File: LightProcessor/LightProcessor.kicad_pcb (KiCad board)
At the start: 2 copper layers, 78.5 x 80.8 mm, 30 parts, among them IC1 STM32G474RET6, J1 USB_C_Receptacle_USB2.0_16P, SW10 Tactile_6mm, U1 STLINK-V3MODS, U3 AP2112K-3.3, Y1 16MHz

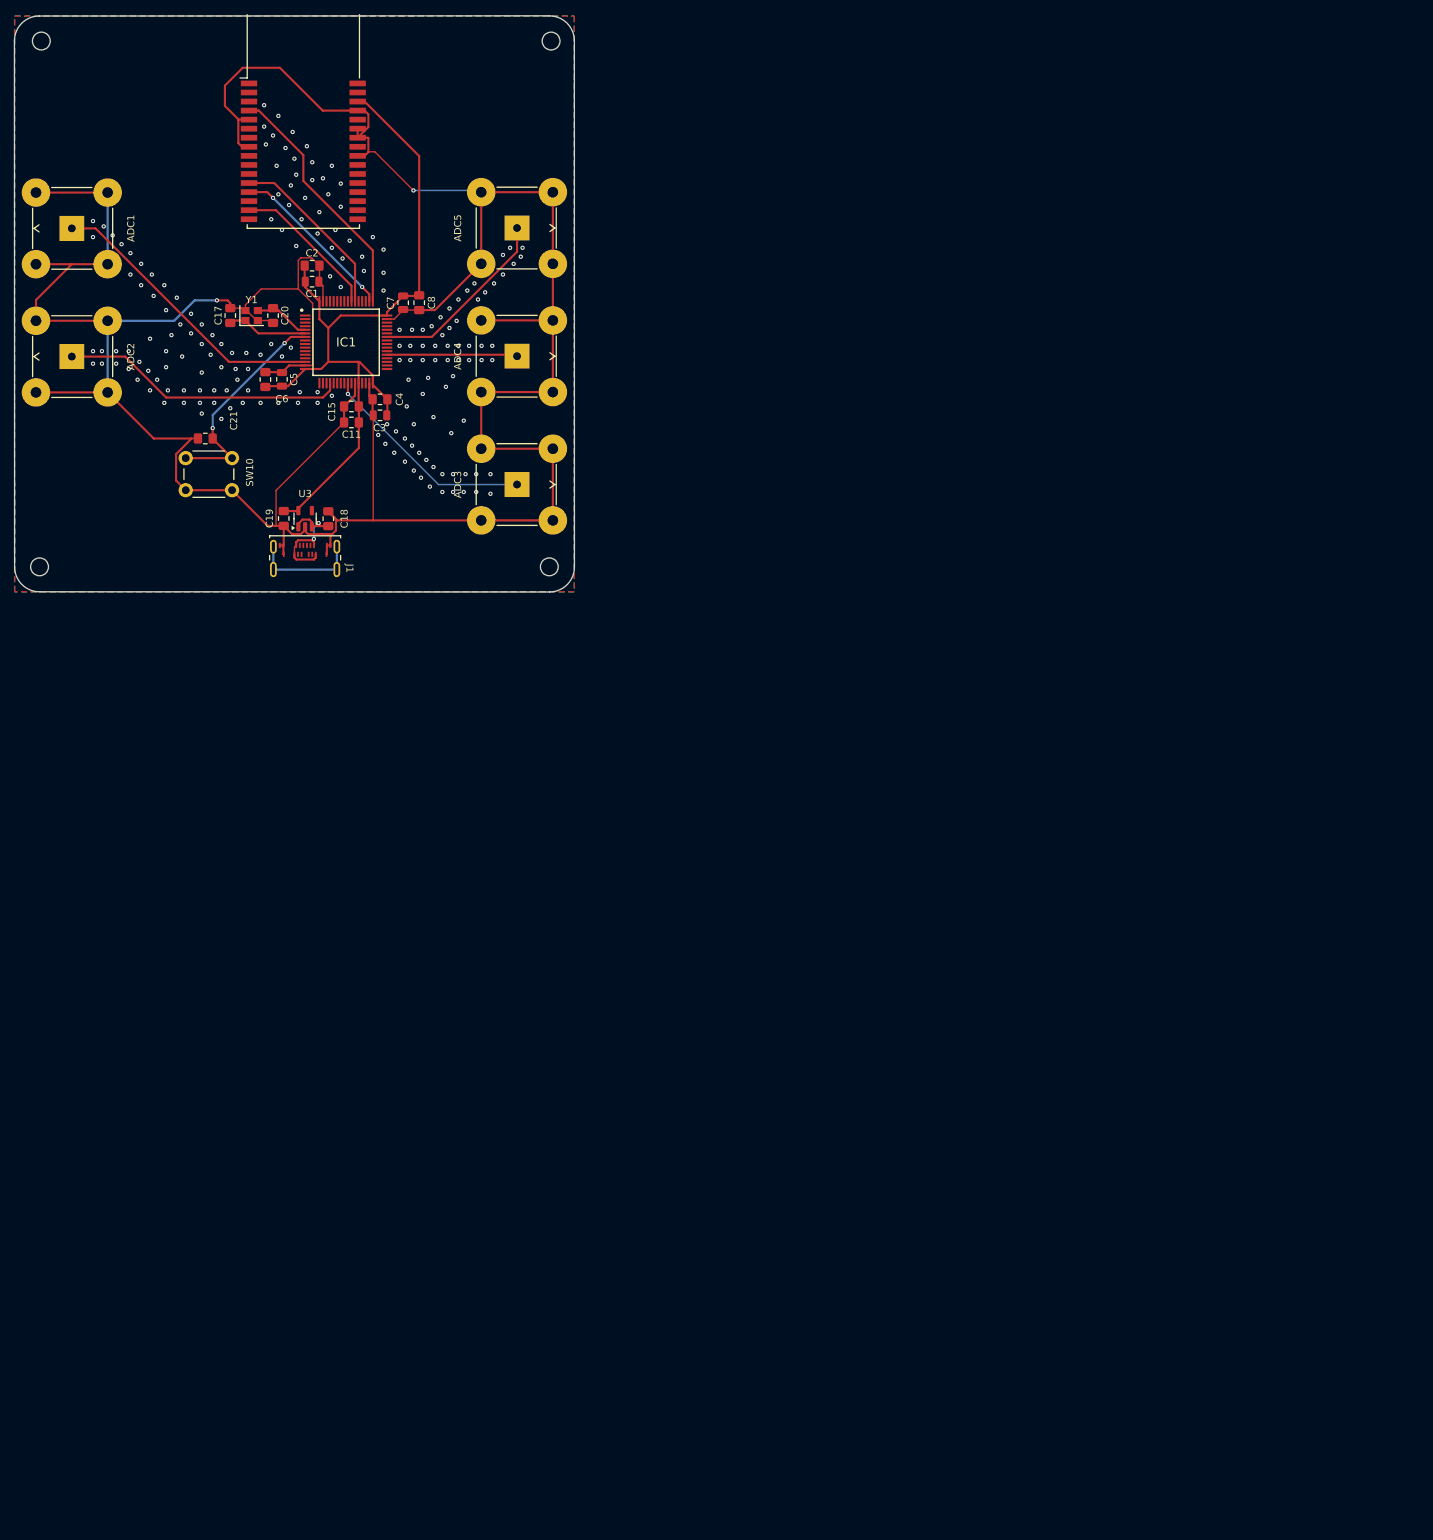
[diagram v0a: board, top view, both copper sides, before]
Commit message: Update PCB design
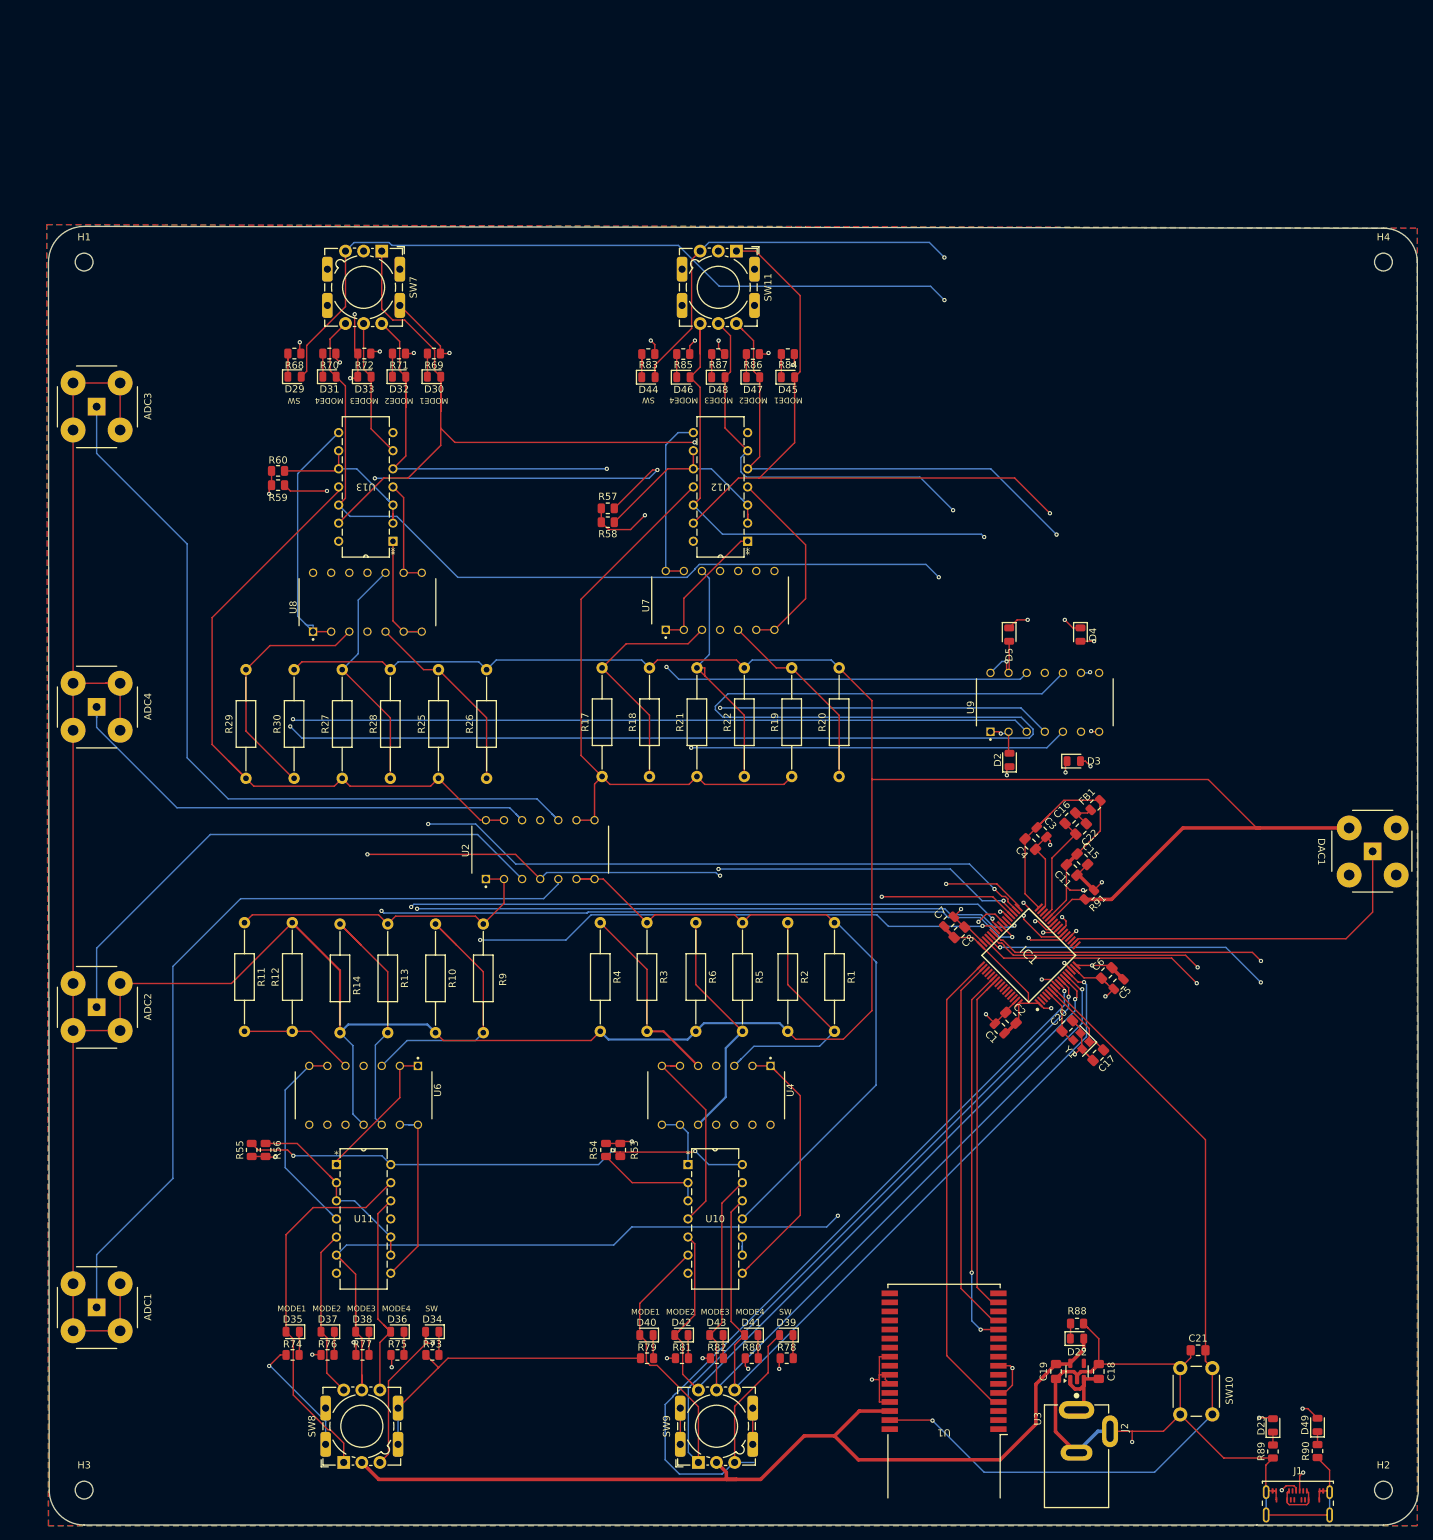
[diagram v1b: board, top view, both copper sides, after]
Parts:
- removed ADC5: Conn_Coaxial, Connector_Coaxial:BNC_TEConnectivity_1478035_Horizontal
- added C16: 0.1, Capacitor_SMD:C_0805_2012Metric_Pad1.18x1.45mm_HandSolder, F.Cu at (254.9, 150.7)
- added C22: 0.1u, Capacitor_SMD:C_0805_2012Metric_Pad1.18x1.45mm_HandSolder, F.Cu at (256.4, 152.2)
- added D2: D, Diode_SMD:D_0805_2012Metric, F.Cu at (246.3, 142.5)
- added D22: LED, LED_SMD:LED_0805_2012Metric, F.Cu at (255.8, 223.7)
- added D23: RED, LED_SMD:LED_0805_2012Metric, F.Cu at (283.3, 235.8)
- added D29: RED, LED_SMD:LED_0805_2012Metric, F.Cu at (146.0, 88.8)
- added D3: D, Diode_SMD:D_0805_2012Metric, F.Cu at (255.3, 142.7)
- added D30: LED, LED_SMD:LED_0805_2012Metric, F.Cu at (165.6, 88.8)
- added D31: LED, LED_SMD:LED_0805_2012Metric, F.Cu at (150.9, 88.8)
- added D32: LED, LED_SMD:LED_0805_2012Metric, F.Cu at (160.7, 88.8)
- added D33: LED, LED_SMD:LED_0805_2012Metric, F.Cu at (155.8, 88.8)
- added D34: RED, LED_SMD:LED_0805_2012Metric, F.Cu at (165.4, 222.7)
- added D35: LED, LED_SMD:LED_0805_2012Metric, F.Cu at (145.8, 222.7)
- added D36: LED, LED_SMD:LED_0805_2012Metric, F.Cu at (160.5, 222.7)
- added D37: LED, LED_SMD:LED_0805_2012Metric, F.Cu at (150.7, 222.7)
- added D38: LED, LED_SMD:LED_0805_2012Metric, F.Cu at (155.5, 222.7)
- added D39: RED, LED_SMD:LED_0805_2012Metric, F.Cu at (215.0, 223.2)
- added D4: D, Diode_SMD:D_0805_2012Metric, F.Cu at (256.3, 124.9)
- added D40: LED, LED_SMD:LED_0805_2012Metric, F.Cu at (195.4, 223.2)
- added D41: LED, LED_SMD:LED_0805_2012Metric, F.Cu at (210.1, 223.2)
- added D42: LED, LED_SMD:LED_0805_2012Metric, F.Cu at (200.3, 223.2)
- added D43: LED, LED_SMD:LED_0805_2012Metric, F.Cu at (205.2, 223.2)
- added D44: RED, LED_SMD:LED_0805_2012Metric, F.Cu at (195.7, 88.8)
- added D45: LED, LED_SMD:LED_0805_2012Metric, F.Cu at (215.3, 88.8)
- added D46: LED, LED_SMD:LED_0805_2012Metric, F.Cu at (200.6, 88.8)
- added D47: LED, LED_SMD:LED_0805_2012Metric, F.Cu at (210.3, 88.8)
- added D48: LED, LED_SMD:LED_0805_2012Metric, F.Cu at (205.5, 88.8)
- added D49: GREEN, LED_SMD:LED_0805_2012Metric, F.Cu at (289.5, 235.8)
- added D5: D, Diode_SMD:D_0805_2012Metric, F.Cu at (246.3, 124.9)
- added DAC1: Conn_Coaxial, 5415025-2:CONN BNC JACK RA 50 OHM PCB, F.Cu at (297.3, 155.3)
- added FB1: FerriteBead, Capacitor_SMD:C_0805_2012Metric, F.Cu at (258.4, 148.8)
- added J2: PJ-202B, PJ_202B:CUI_PJ-202B, F.Cu at (255.7, 240.2)
- added R1: 500K, Resistor_THT:R_Axial_DIN0207_L6.3mm_D2.5mm_P15.24mm_Horizontal, F.Cu at (221.8, 165.3)
- added R10: 330K, Resistor_THT:R_Axial_DIN0207_L6.3mm_D2.5mm_P15.24mm_Horizontal, F.Cu at (165.8, 165.5)
- added R11: 1M, Resistor_THT:R_Axial_DIN0207_L6.3mm_D2.5mm_P15.24mm_Horizontal, F.Cu at (139.0, 165.3)
- added R12: 330K, Resistor_THT:R_Axial_DIN0207_L6.3mm_D2.5mm_P15.24mm_Horizontal, F.Cu at (145.7, 180.6)
- added R13: 250K, Resistor_THT:R_Axial_DIN0207_L6.3mm_D2.5mm_P15.24mm_Horizontal, F.Cu at (159.1, 165.5)
- added R14: 110K, Resistor_THT:R_Axial_DIN0207_L6.3mm_D2.5mm_P15.24mm_Horizontal, F.Cu at (152.4, 165.5)
- added R17: 500K, Resistor_THT:R_Axial_DIN0207_L6.3mm_D2.5mm_P15.24mm_Horizontal, F.Cu at (189.2, 144.8)
- added R18: 330K, Resistor_THT:R_Axial_DIN0207_L6.3mm_D2.5mm_P15.24mm_Horizontal, F.Cu at (195.8, 144.8)
- added R19: 1M, Resistor_THT:R_Axial_DIN0207_L6.3mm_D2.5mm_P15.24mm_Horizontal, F.Cu at (215.8, 144.8)
- added R2: 330K, Resistor_THT:R_Axial_DIN0207_L6.3mm_D2.5mm_P15.24mm_Horizontal, F.Cu at (215.2, 165.3)
- added R20: 330K, Resistor_THT:R_Axial_DIN0207_L6.3mm_D2.5mm_P15.24mm_Horizontal, F.Cu at (222.4, 144.8)
- added R21: 250K, Resistor_THT:R_Axial_DIN0207_L6.3mm_D2.5mm_P15.24mm_Horizontal, F.Cu at (202.5, 144.8)
- added R22: 110K, Resistor_THT:R_Axial_DIN0207_L6.3mm_D2.5mm_P15.24mm_Horizontal, F.Cu at (209.1, 144.8)
- added R25: 500K, Resistor_THT:R_Axial_DIN0207_L6.3mm_D2.5mm_P15.24mm_Horizontal, F.Cu at (166.2, 145.1)
- added R26: 330K, Resistor_THT:R_Axial_DIN0207_L6.3mm_D2.5mm_P15.24mm_Horizontal, F.Cu at (173.0, 145.1)
- added R27: 1M, Resistor_THT:R_Axial_DIN0207_L6.3mm_D2.5mm_P15.24mm_Horizontal, F.Cu at (152.7, 145.1)
- added R28: 330K, Resistor_THT:R_Axial_DIN0207_L6.3mm_D2.5mm_P15.24mm_Horizontal, F.Cu at (159.5, 145.1)
- added R29: 250K, Resistor_THT:R_Axial_DIN0207_L6.3mm_D2.5mm_P15.24mm_Horizontal, F.Cu at (139.2, 145.1)
- added R3: 1M, Resistor_THT:R_Axial_DIN0207_L6.3mm_D2.5mm_P15.24mm_Horizontal, F.Cu at (195.5, 165.3)
- added R30: 110K, Resistor_THT:R_Axial_DIN0207_L6.3mm_D2.5mm_P15.24mm_Horizontal, F.Cu at (146.0, 145.1)
- added R4: 330K, Resistor_THT:R_Axial_DIN0207_L6.3mm_D2.5mm_P15.24mm_Horizontal, F.Cu at (188.9, 165.3)
- added R5: 250K, Resistor_THT:R_Axial_DIN0207_L6.3mm_D2.5mm_P15.24mm_Horizontal, F.Cu at (208.9, 165.3)
- added R53: 100K, Resistor_SMD:R_0805_2012Metric, F.Cu at (191.7, 197.2)
- added R54: 100K, Resistor_SMD:R_0805_2012Metric, F.Cu at (189.7, 197.2)
- added R55: 100K, Resistor_SMD:R_0805_2012Metric, F.Cu at (140.0, 197.2)
- added R56: 100K, Resistor_SMD:R_0805_2012Metric, F.Cu at (142.0, 197.2)
- added R57: 100K, Resistor_SMD:R_0805_2012Metric, F.Cu at (190.0, 107.2)
- added R58: 100K, Resistor_SMD:R_0805_2012Metric, F.Cu at (190.0, 109.2)
- added R59: 100K, Resistor_SMD:R_0805_2012Metric, F.Cu at (143.7, 104.0)
- added R6: 110K, Resistor_THT:R_Axial_DIN0207_L6.3mm_D2.5mm_P15.24mm_Horizontal, F.Cu at (202.3, 165.3)
- added R60: 100K, Resistor_SMD:R_0805_2012Metric, F.Cu at (143.7, 102.0)
- added R68: 100K, Resistor_SMD:R_0805_2012Metric, F.Cu at (146.0, 85.5)
- added R69: 100K, Resistor_SMD:R_0805_2012Metric, F.Cu at (165.6, 85.5)
- added R70: 100K, Resistor_SMD:R_0805_2012Metric, F.Cu at (150.9, 85.5)
- added R71: 100K, Resistor_SMD:R_0805_2012Metric, F.Cu at (160.7, 85.5)
- added R72: 100K, Resistor_SMD:R_0805_2012Metric, F.Cu at (155.8, 85.5)
- added R73: 100K, Resistor_SMD:R_0805_2012Metric, F.Cu at (165.4, 226.0)
- added R74: 100K, Resistor_SMD:R_0805_2012Metric, F.Cu at (145.8, 226.0)
- added R75: 100K, Resistor_SMD:R_0805_2012Metric, F.Cu at (160.5, 226.0)
- added R76: 100K, Resistor_SMD:R_0805_2012Metric, F.Cu at (150.7, 226.0)
- added R77: 100K, Resistor_SMD:R_0805_2012Metric, F.Cu at (155.6, 226.0)
- added R78: 100K, Resistor_SMD:R_0805_2012Metric, F.Cu at (215.1, 226.4)
- added R79: 100K, Resistor_SMD:R_0805_2012Metric, F.Cu at (195.5, 226.4)
- added R80: 100K, Resistor_SMD:R_0805_2012Metric, F.Cu at (210.2, 226.4)
- added R81: 100K, Resistor_SMD:R_0805_2012Metric, F.Cu at (200.4, 226.4)
- added R82: 100K, Resistor_SMD:R_0805_2012Metric, F.Cu at (205.3, 226.4)
- added R83: 100K, Resistor_SMD:R_0805_2012Metric, F.Cu at (195.7, 85.6)
- added R84: 100K, Resistor_SMD:R_0805_2012Metric, F.Cu at (215.2, 85.6)
- added R85: 100K, Resistor_SMD:R_0805_2012Metric, F.Cu at (200.6, 85.6)
- added R86: 100K, Resistor_SMD:R_0805_2012Metric, F.Cu at (210.3, 85.6)
- added R87: 100K, Resistor_SMD:R_0805_2012Metric, F.Cu at (205.5, 85.6)
- added R88: 100K, Resistor_SMD:R_0805_2012Metric, F.Cu at (255.8, 221.6)
- added R89: 100K, Resistor_SMD:R_0805_2012Metric, F.Cu at (283.3, 239.5)
- added R9: 500K, Resistor_THT:R_Axial_DIN0207_L6.3mm_D2.5mm_P15.24mm_Horizontal, F.Cu at (172.5, 165.5)
- added R90: 100K, Resistor_SMD:R_0805_2012Metric, F.Cu at (289.5, 239.4)
- added R91: 0, Resistor_SMD:R_0805_2012Metric, F.Cu at (257.5, 161.4)
- added SW11: SW_SP5T_NR01105, Button_Switch_THT:SW_NKK_NR01, F.Cu at (208.0, 71.1)
- added SW7: SW_SP5T_NR01105, Button_Switch_THT:SW_NKK_NR01, F.Cu at (158.3, 71.1)
- added SW8: SW_SP5T_NR01105, Button_Switch_THT:SW_NKK_NR01, F.Cu at (152.9, 241.0)
- added SW9: SW_SP5T_NR01105, Button_Switch_THT:SW_NKK_NR01, F.Cu at (202.7, 241.0)
- added U10: SN74HC4066N, SN74HC4066N:N14, F.Cu at (208.8, 214.5)
- added U11: SN74HC4066N, SN74HC4066N:N14, F.Cu at (159.5, 214.5)
- added U12: SN74HC4066N, SN74HC4066N:N14, F.Cu at (202.0, 96.6)
- added U13: SN74HC4066N, SN74HC4066N:N14, F.Cu at (152.2, 96.6)
- added U2: LM324, LM324N_NOPB:DIP825W47P254L1917H533Q14, F.Cu at (180.5, 155.1)
- added U4: LM324, LM324N_NOPB:DIP825W47P254L1917H533Q14, F.Cu at (205.2, 189.6)
- added U6: LM324, LM324N_NOPB:DIP825W47P254L1917H533Q14, F.Cu at (155.7, 189.6)
- added U7: LM324, LM324N_NOPB:DIP825W47P254L1917H533Q14, F.Cu at (205.7, 120.1)
- added U8: LM324, LM324N_NOPB:DIP825W47P254L1917H533Q14, F.Cu at (156.3, 120.4)
- added U9: LM324, LM324N_NOPB:DIP825W47P254L1917H533Q14, F.Cu at (251.3, 134.4)
- ADC1, ADC2, ADC3, ADC4: footprint Connector_Coaxial:BNC_TEConnectivity_1478035_Horizontal -> 5415025-2:CONN BNC JACK RA 50 OHM PCB
- C11: value 1u -> 0.1u
- moved H3 213.5 mm to (116.5, 244.9)
- moved U1 209.1 mm to (237.1, 236.4), turned to 180 degrees
- moved J1 192.3 mm to (286.8, 248.2)
- moved H4 190.8 mm to (298.8, 72.7)
- moved C21 189.1 mm to (272.8, 225.3)
- moved SW10 185.7 mm to (270.3, 234.3), turned to 90 degrees
- moved H2 174.5 mm to (298.8, 244.9)
- moved C19 161.4 mm to (252.9, 228.3)
- moved U3 161.3 mm to (255.8, 228.3)
- moved C18 161.2 mm to (258.9, 228.3)
- moved C17 160.0 mm to (258.8, 183.9), turned to -135 degrees
- moved Y1 154.6 mm to (256.4, 181.9), turned to 135 degrees
- moved ADC1 151.4 mm to (118.3, 219.3)
- moved C20 149.5 mm to (254.4, 179.8), turned to 45 degrees
- moved C5 144.8 mm to (261.6, 174.0), turned to 45 degrees
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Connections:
- ADC1 pad 1: /ADC1_IN3 -> /ADC1_RAW
- ADC1 pad 2: GND -> AGND
- ADC2 pad 1: /ADC2_IN3 -> /ADC2_RAW
- ADC2 pad 2: GND -> AGND
- ADC3 pad 1: /ADC3_IN1 -> /ADC3_RAW
- ADC3 pad 2: GND -> AGND
- ADC4 pad 1: /ADC4_IN5 -> /ADC4_RAW
- ADC4 pad 2: GND -> AGND
- IC1 pad 1: unconnected-(IC1-VBAT-Pad1) -> +3.3V
- IC1 pad 10: unconnected-(IC1-PC2-Pad10) -> /ADC1_MOD1_IND
- IC1 pad 11: unconnected-(IC1-PC3-Pad11) -> /ADC1_MOD2_IND
- IC1 pad 12: unconnected-(IC1-PA0-Pad12) -> /ADC1_MOD3_IND
- IC1 pad 13: unconnected-(IC1-PA1-Pad13) -> /ADC1_MOD4_IND
- IC1 pad 14: /ADC1_IN3 -> Net-(D3-K)
- IC1 pad 18: unconnected-(IC1-PA4-Pad18) -> /DAC_OUT
- IC1 pad 20: /ADC2_IN3 -> Net-(D4-K)
- IC1 pad 21: unconnected-(IC1-PA7-Pad21) -> /ADC3_MOD4_IND
- IC1 pad 22: unconnected-(IC1-PC4-Pad22) -> /ADC3_MOD3_IND
- IC1 pad 23: unconnected-(IC1-PC5-Pad23) -> /ADC3_MOD2_IND
- IC1 pad 24: unconnected-(IC1-PB0-Pad24) -> /ADC3_MOD1_IND
- IC1 pad 25: /ADC3_IN1 -> Net-(D5-K)
- IC1 pad 26: unconnected-(IC1-PB2-Pad26) -> /ADC3_IDLE_IND
- IC1 pad 27: GND -> AGND
- IC1 pad 29: unconnected-(IC1-VDDA-Pad29) -> Net-(IC1-VDDA)
- IC1 pad 33: unconnected-(IC1-PB11-Pad33) -> /ADC4_MOD4_IND
- IC1 pad 34: unconnected-(IC1-PB12-Pad34) -> /ADC4_MOD3_IND
- IC1 pad 35: unconnected-(IC1-PB13-Pad35) -> /ADC4_MOD2_IND
- IC1 pad 36: unconnected-(IC1-PB14-Pad36) -> /ADC4_MOD1_IND
- IC1 pad 37: /ADC4_IN5 -> Net-(D2-K)
- IC1 pad 38: unconnected-(IC1-PC6-Pad38) -> /ADC2_MOD4_IND
- IC1 pad 39: unconnected-(IC1-PC7-Pad39) -> /ADC2_MOD3_IND
- IC1 pad 40: unconnected-(IC1-PC8-Pad40) -> /ADC2_MOD2_IND
- IC1 pad 41: unconnected-(IC1-PC9-Pad41) -> /ADC2_MOD1_IND
- IC1 pad 42: /ADC5_IN1 -> /ADC2_IDLE_IND
- IC1 pad 43: unconnected-(IC1-PA9-Pad43) -> /RX_IND
- IC1 pad 44: unconnected-(IC1-PA10-Pad44) -> /TX_IND
- IC1 pad 45: unconnected-(IC1-PA11-Pad45) -> /D-
- IC1 pad 46: unconnected-(IC1-PA12-Pad46) -> /D+
- IC1 pad 51: /PA15 -> unconnected-(IC1-PA15-Pad51)
- IC1 pad 52: /PC10 -> unconnected-(IC1-PC10-Pad52)
- IC1 pad 53: /PC11 -> unconnected-(IC1-PC11-Pad53)
- IC1 pad 56: /PB3 -> unconnected-(IC1-PB3-Pad56)
- IC1 pad 57: /PB4 -> unconnected-(IC1-PB4-Pad57)
- IC1 pad 58: /PB5 -> unconnected-(IC1-PB5-Pad58)
- IC1 pad 59: /PB6 -> unconnected-(IC1-PB6-Pad59)
- IC1 pad 60: /PB7 -> unconnected-(IC1-PB7-Pad60)
- IC1 pad 61: /PB8 -> unconnected-(IC1-PB8-BOOT0-Pad61)
- IC1 pad 62: /PB9 -> unconnected-(IC1-PB9-Pad62)
- IC1 pad 8: unconnected-(IC1-PC0-Pad8) -> /ADC4_IDLE_IND
- IC1 pad 9: unconnected-(IC1-PC1-Pad9) -> /ADC1_IDLE_IND
- J1 pad A4: +5V -> Net-(J1-VBUS-PadA4)
- J1 pad A6: unconnected-(J1-D+-PadA6) -> /D+
- J1 pad A7: unconnected-(J1-D--PadA7) -> /D-
- J1 pad A9: +5V -> Net-(J1-VBUS-PadA4)
- J1 pad B4: +5V -> Net-(J1-VBUS-PadA4)
- J1 pad B9: +5V -> Net-(J1-VBUS-PadA4)
- J1 pad S1: unconnected-(J1-SHIELD-PadS1) -> GND
- U1 pad 31: unconnected-(U1-NRST-Pad31) -> /~{RESET}
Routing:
- net AGND: track 0.00 -> 691.6 mm
- net +3.3V: track 112.6 -> 684.5 mm, vias 0 -> 10
- net +5V: track 19.1 -> 328.4 mm, vias 2 -> 3
- net Net-(U9C-+): track 0.00 -> 267.3 mm, vias 0 -> 2
- net /ADC4_IDLE_IND: track 0.00 -> 211.8 mm, vias 0 -> 2
- net /ADC4_MOD1_IND: track 0.00 -> 185.6 mm, vias 0 -> 2
- net /ADC2_MOD1_IND: track 0.00 -> 178.1 mm, vias 0 -> 2
- net /ADC4_MOD4_IND: track 0.00 -> 172.7 mm, vias 0 -> 2
- net /ADC2_MOD2_IND: track 0.00 -> 165.1 mm, vias 0 -> 2
- net /ADC4_MOD2_IND: track 0.00 -> 163.5 mm, vias 0 -> 3
- net /ADC4_MOD3_IND: track 0.00 -> 162.3 mm, vias 0 -> 2
- net /ADC2_MOD4_IND: track 0.00 -> 159.3 mm, vias 0 -> 2
- net GND: track 461.6 -> 302.4 mm, vias 187 -> 27
- net /ADC3_IDLE_IND: track 0.00 -> 158.4 mm, vias 0 -> 2
- net /ADC2_IDLE_IND: track 0.00 -> 157.9 mm, vias 0 -> 3
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- added copper zone on In1.Cu, net GND
- added copper zone on In2.Cu, net GND
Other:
- board size 78.5 x 80.8 mm -> 192.1 x 182.1 mm
- copper layers 2 -> 4
- board text added: "MODE1"
- board text added: "MODE2"
- board text added: "MODE3"
- board text added: "MODE4"
- board text added: "SW"
